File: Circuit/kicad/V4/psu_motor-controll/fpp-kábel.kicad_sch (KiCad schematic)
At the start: 9 parts, among them J5 Conn_01x60_MountingPin

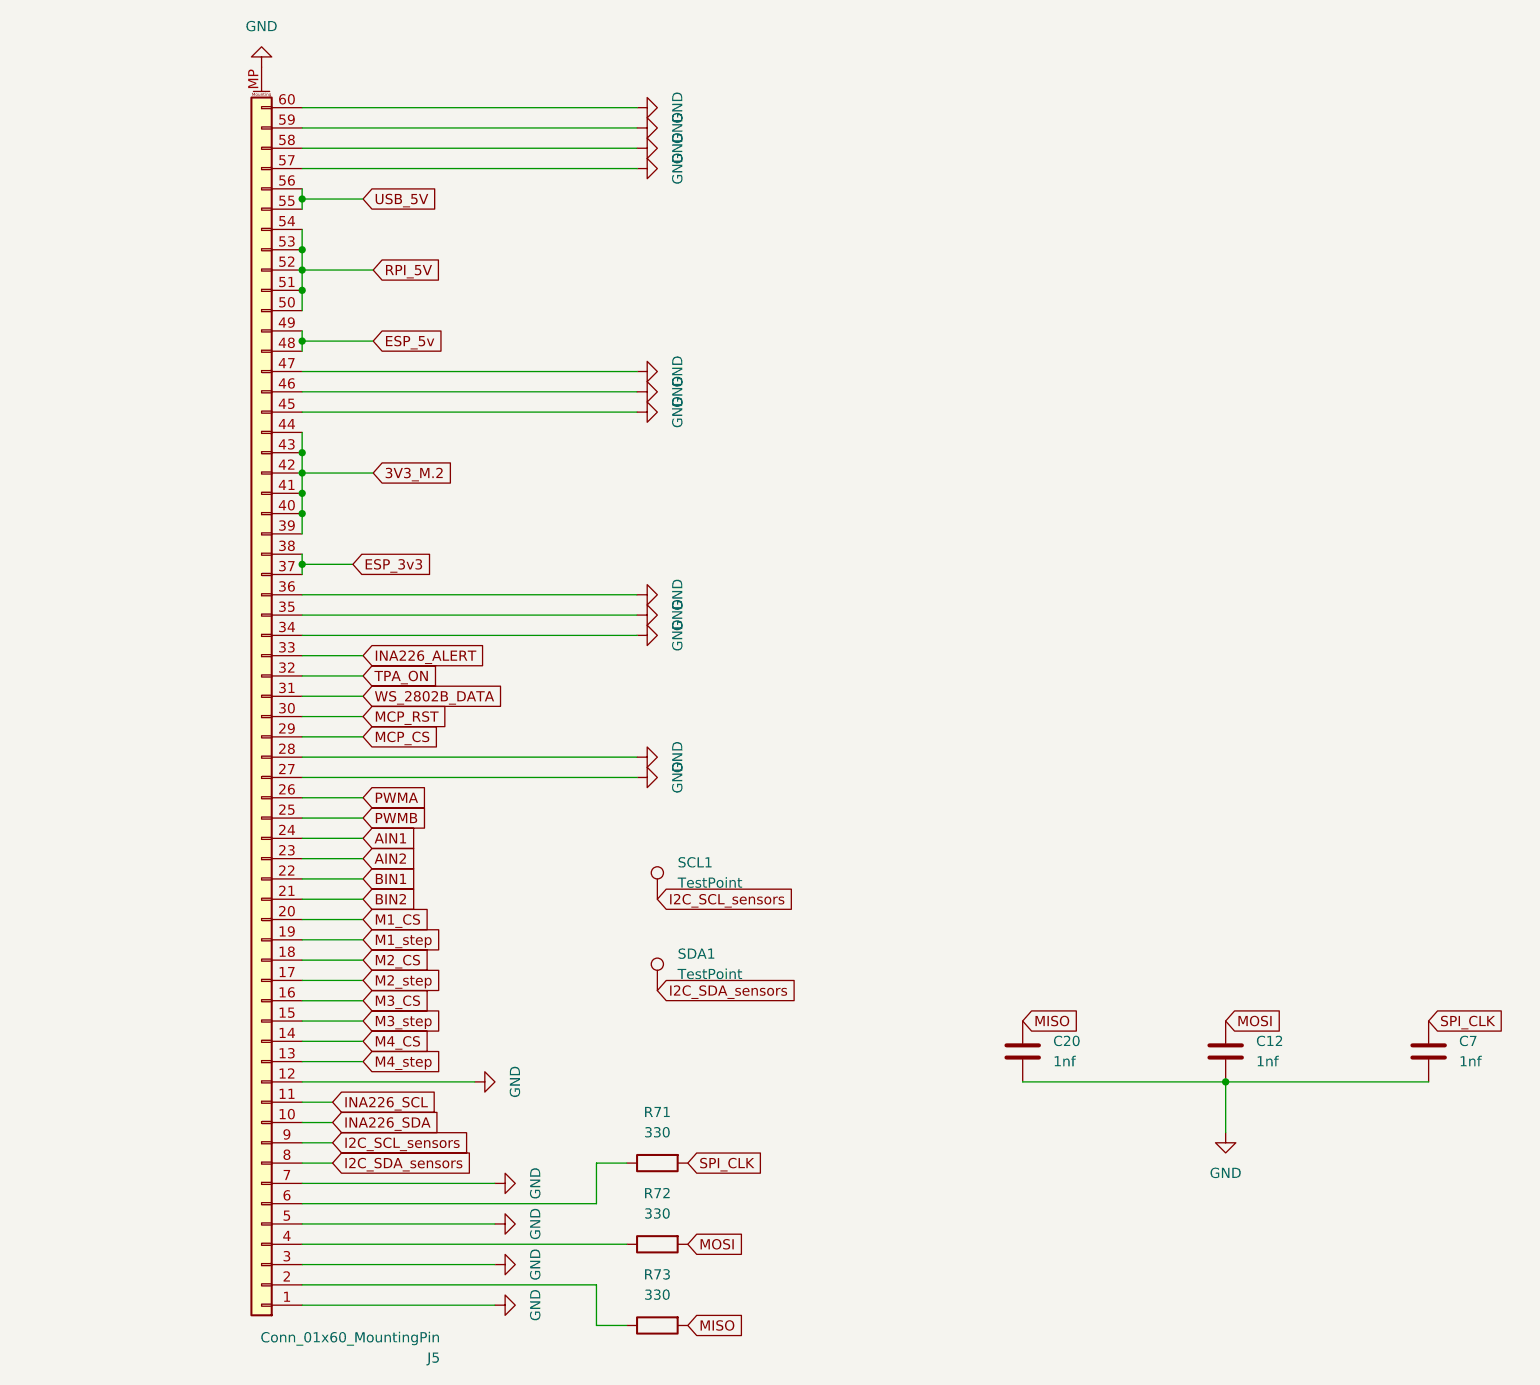
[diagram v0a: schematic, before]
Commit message: kicad
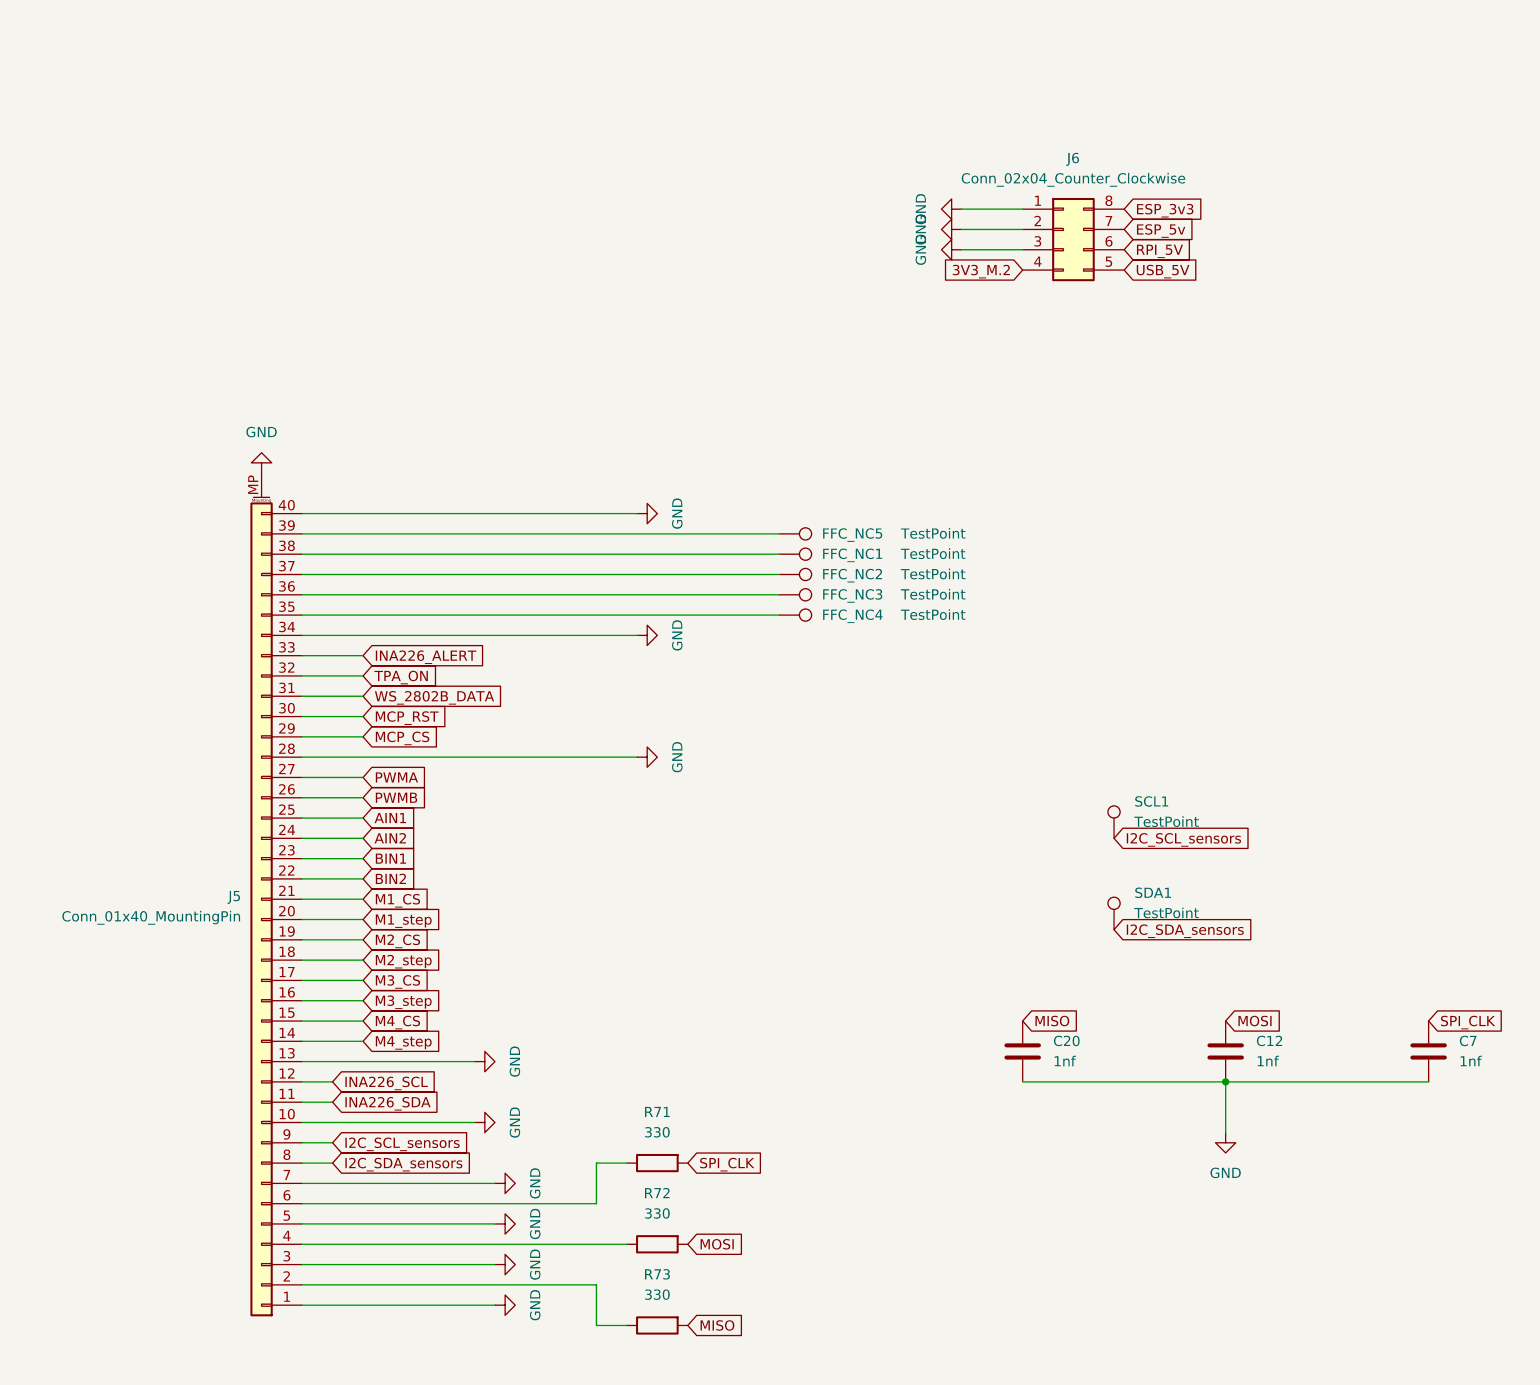
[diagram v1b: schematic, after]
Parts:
- removed J5: Conn_01x60_MountingPin, Connector_FFC-FPC:Amphenol_F32Q-1A7x1-11060_1x60-1MP_P0.5mm_Horizontal, symbol Connector_Generic_MountingPin:Conn_01x60_MountingPin
- added FFC_NC1, FFC_NC2, FFC_NC3, FFC_NC4, FFC_NC5: TestPoint, TestPoint:TestPoint_Pad_D1.0mm, symbol Connector:TestPoint
- added J5: Conn_01x40_MountingPin, Connector_FFC-FPC:Amphenol_F32Q-1A7x1-11040_1x40-1MP_P0.5mm_Horizontal, symbol Connector_Generic_MountingPin:Conn_01x40_MountingPin
- added J6: Conn_02x04_Counter_Clockwise, Connector_Molex:Molex_Micro-Fit_3.0_43045-0812_2x04_P3.00mm_Vertical, symbol Connector_Generic:Conn_02x04_Counter_Clockwise
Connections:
- net 3V3_M.2: now also J6.4 (Pin_4)
- net AIN1: now also J5.25 (Pin_25)
- net AIN2: now also J5.24 (Pin_24)
- net BIN1: now also J5.23 (Pin_23)
- net BIN2: now also J5.22 (Pin_22)
- net ESP_3v3: now also J6.8 (Pin_8)
- net ESP_5v: now also J6.7 (Pin_7)
- net GND: now also J5.1 (Pin_1), J5.10 (Pin_10), J5.13 (Pin_13), J5.28 (Pin_28), J5.3 (Pin_3), J5.34 (Pin_34), J5.40 (Pin_40), J5.5 (Pin_5), J5.7 (Pin_7), J5.MP (MountPin), J6.1 (Pin_1), J6.2 (Pin_2), J6.3 (Pin_3)
- net I2C_SCL_sensors: now also J5.9 (Pin_9)
- net I2C_SDA_sensors: now also J5.8 (Pin_8)
- net INA226_ALERT: now also J5.33 (Pin_33)
- net INA226_SCL: now also J5.12 (Pin_12)
- net INA226_SDA: now also J5.11 (Pin_11)
- net M1_CS: now also J5.21 (Pin_21)
- net M1_step: now also J5.20 (Pin_20)
- net M2_CS: now also J5.19 (Pin_19)
- net M2_step: now also J5.18 (Pin_18)
- net M3_CS: now also J5.17 (Pin_17)
- net M3_step: now also J5.16 (Pin_16)
- net M4_CS: now also J5.15 (Pin_15)
- net M4_step: now also J5.14 (Pin_14)
- net MCP_CS: now also J5.29 (Pin_29)
- net MCP_RST: now also J5.30 (Pin_30)
- net PWMA: now also J5.27 (Pin_27)
- net PWMB: now also J5.26 (Pin_26)
- net RPI_5V: now also J6.6 (Pin_6)
- net TPA_ON: now also J5.32 (Pin_32)
- net USB_5V: now also J6.5 (Pin_5)
- net WS_2802B_DATA: now also J5.31 (Pin_31)
- net at R72.1: now also J5.4 (Pin_4)
- net at R73.1: now also J5.2 (Pin_2)
- net at R71.1: now also J5.6 (Pin_6)
- new net: FFC_NC2.1, J5.37 (Pin_37)
- new net: FFC_NC1.1, J5.38 (Pin_38)
- new net: FFC_NC5.1, J5.39 (Pin_39)
- new net: FFC_NC3.1, J5.36 (Pin_36)
- new net: FFC_NC4.1, J5.35 (Pin_35)
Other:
- moved on the sheet: SCL1, SDA1
